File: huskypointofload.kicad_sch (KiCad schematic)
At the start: 8 parts, among them J1 POWER, J2 RFSOC_POWER

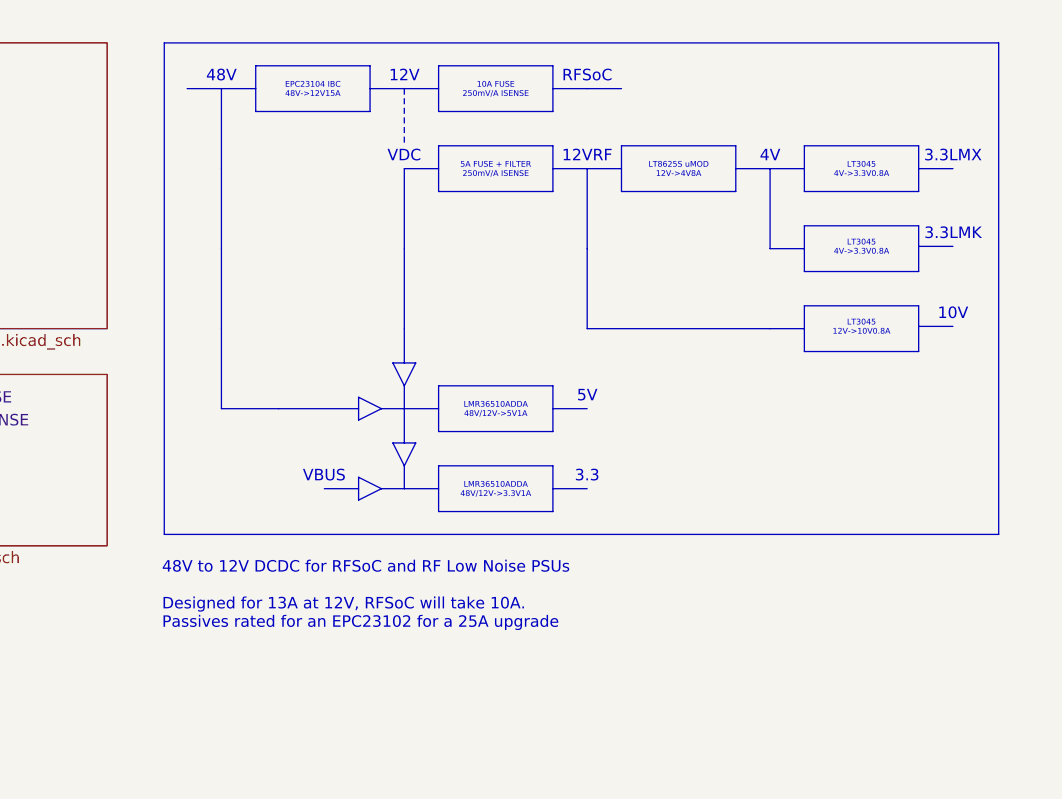
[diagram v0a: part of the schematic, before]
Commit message: Add LMX Draft
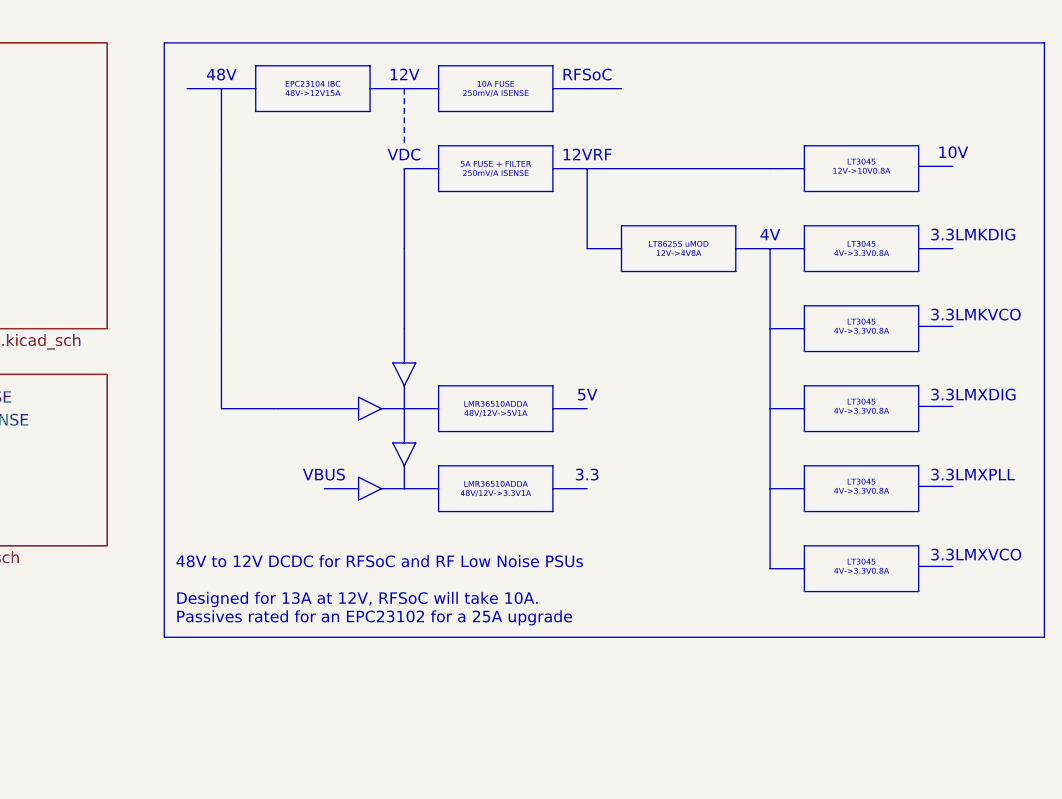
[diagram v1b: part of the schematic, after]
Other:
- note added: "3.3LMKDIG"
- note added: "3.3LMKVCO"
- note added: "3.3LMXDIG"
- note added: "3.3LMXPLL"
- note added: "3.3LMXVCO"
- note removed: "3.3LMK"
- note removed: "3.3LMX"
